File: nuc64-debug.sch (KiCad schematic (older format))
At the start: 8 parts, among them J1 SWD, J2 POW, SW1 BOOT, SW2 RST

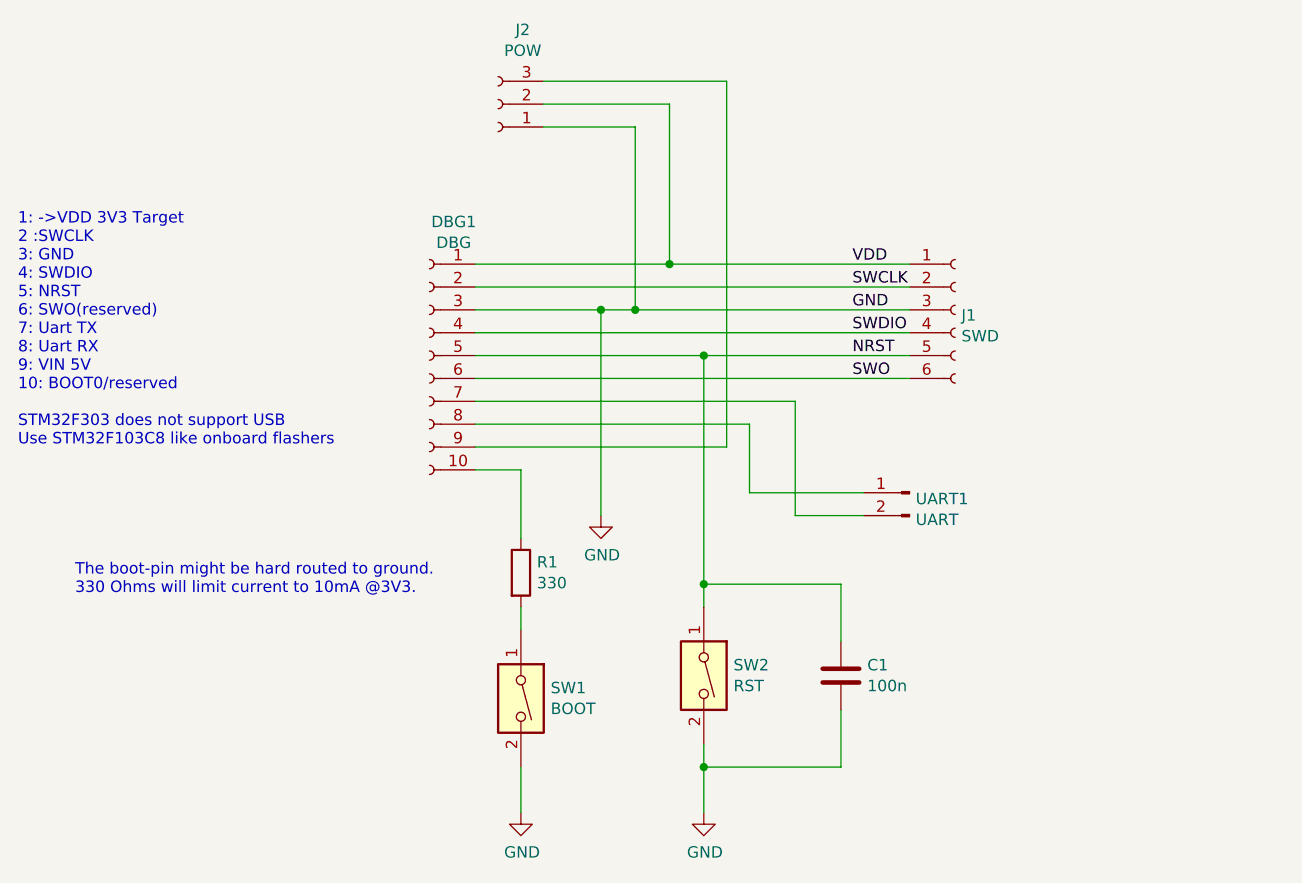
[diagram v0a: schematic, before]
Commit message: shrink
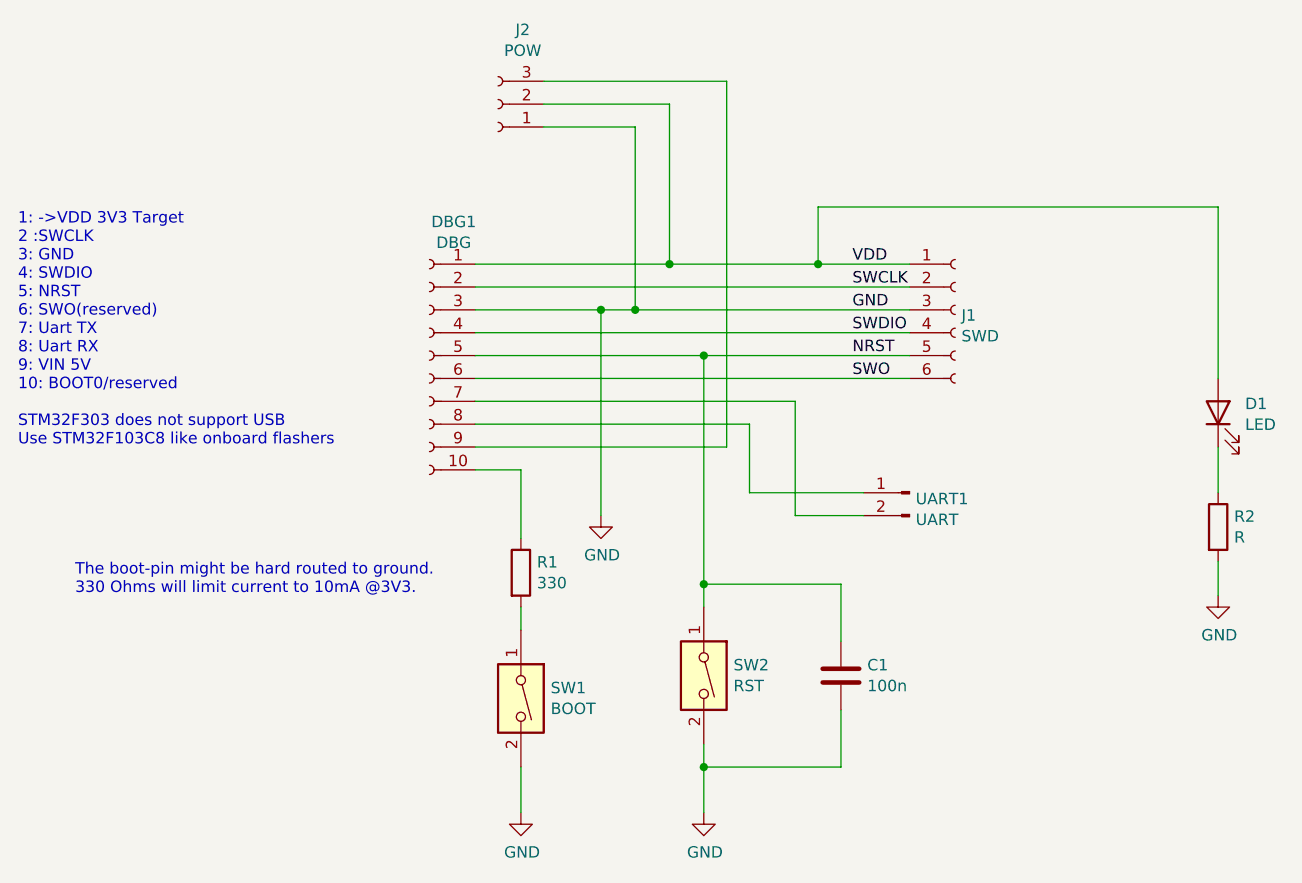
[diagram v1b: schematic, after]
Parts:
- added D1: LED, LED_SMD:LED_0603_1608Metric, symbol Device:LED
- added R2: R, Resistor_SMD:R_0603_1608Metric, symbol Device:R
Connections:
- net GND: now also R2.2
- net VDD: now also D1.2 (A)
- new net: D1.1 (K), R2.1
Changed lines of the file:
@@
 Connection ~ 5750 2200
 Wire Wire Line
-	5750 2200 6800 2200
+	5750 2200 6400 2200
 Wire Wire Line
 	5200 1400 6000 1400
@@
 Wire Wire Line
 	5900 4400 5900 4600
+$Comp
+L power:GND #PWR0104
+U 1 1 60F4062E
+P 8150 3650
+F 0 "#PWR0104" H 8150 3400 50  0001 C CNN
+F 1 "GND" H 8155 3477 50  0000 C CNN
+F 2 "" H 8150 3650 50  0001 C CNN
+F 3 "" H 8150 3650 50  0001 C CNN
+	1    8150 3650
+	1    0    0    -1
+$EndComp
+$Comp
+L Device:R R2
+U 1 1 60F4083F
+P 8150 3350
+F 0 "R2" H 8220 3396 50  0000 L CNN
+F 1 "R" H 8220 3305 50  0000 L CNN
+F 2 "Resistor_SMD:R_0603_1608Metric" V 8080 3350 50  0001 C CNN
+F 3 "~" H 8150 3350 50  0001 C CNN
+	1    8150 3350
+	1    0    0    -1
+$EndComp
+$Comp
+L Device:LED D1
+U 1 1 60F40F26
+P 8150 2850
+F 0 "D1" V 8189 2732 50  0000 R CNN
+F 1 "LED" V 8098 2732 50  0000 R CNN
+F 2 "LED_SMD:LED_0603_1608Metric" H 8150 2850 50  0001 C CNN
+F 3 "~" H 8150 2850 50  0001 C CNN
+	1    8150 2850
+	0    -1   -1   0
+$EndComp
+Wire Wire Line
+	8150 3650 8150 3500
+Wire Wire Line
+	8150 3200 8150 3000
+Wire Wire Line
+	6400 2200 6400 1950
+Wire Wire Line
+	6400 1950 8150 1950
+Wire Wire Line
+	8150 1950 8150 2700
+Connection ~ 6400 2200
+Wire Wire Line
+	6400 2200 6800 2200
 $EndSCHEMATC
